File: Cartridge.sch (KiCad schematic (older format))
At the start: 1 part, among them J4 Expansion

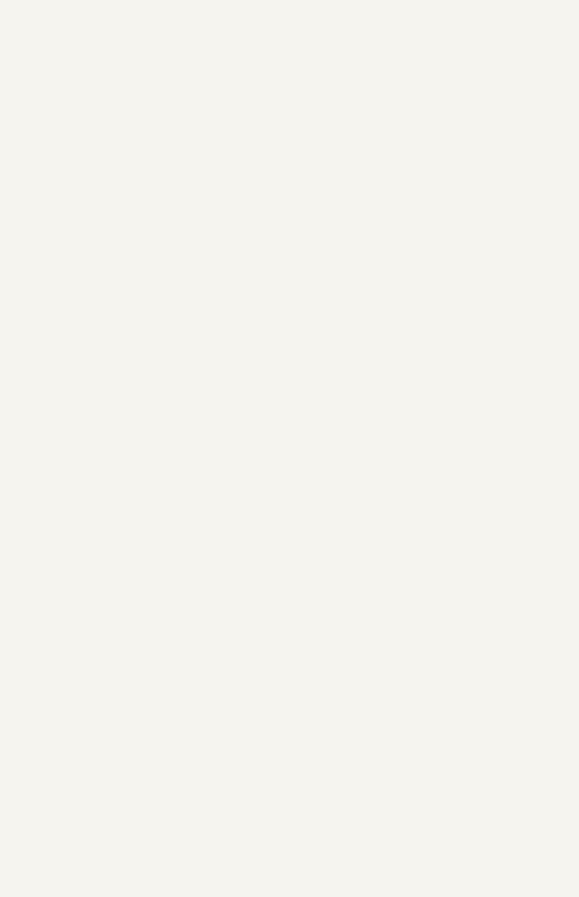
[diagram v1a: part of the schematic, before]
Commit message: MMU, Joy, Cart and Video
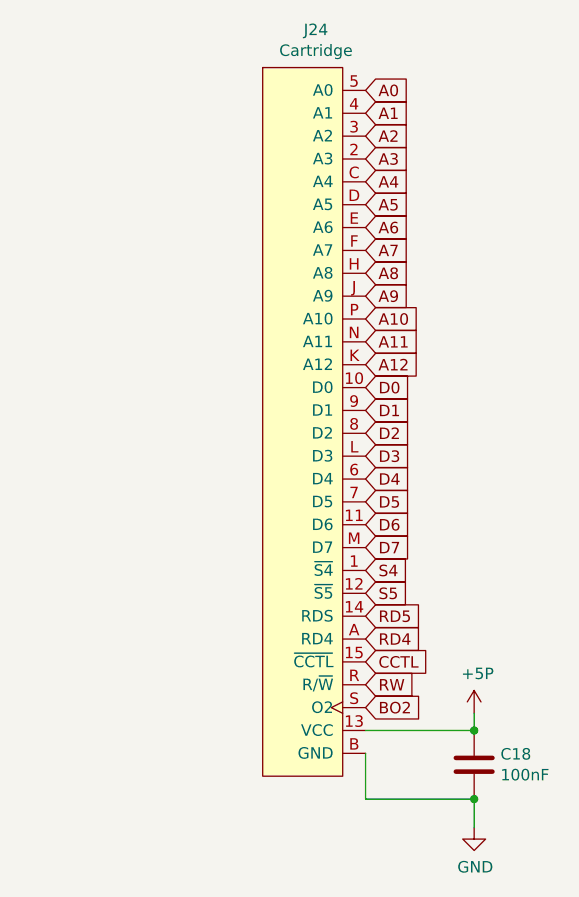
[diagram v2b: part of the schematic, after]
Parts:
- added C18: 100nF, Atari:C_Axial_L5.1mm_D2.5mm_P12.50mm_Horizontal, symbol Device:C
- added J24: Cartridge, Atari:Cartridge_Slot, symbol Atari:Cartridge
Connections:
- net GND: now also C18.2, J24.B (GND)
- new net +5P: C18.1, J24.13 (VCC)
- new net A0: J24.5 (A0)
- new net A1: J24.4 (A1)
- new net A10: J24.P (A10)
- new net A11: J24.N (A11)
- new net A12: J24.K (A12)
- new net A2: J24.3 (A2)
- new net A3: J24.2 (A3)
- new net A4: J24.C (A4)
- new net A5: J24.D (A5)
- new net A6: J24.E (A6)
- new net A7: J24.F (A7)
- new net A8: J24.H (A8)
- new net A9: J24.J (A9)
- new net BO2: J24.S (O2)
- new net CCTL: J24.15 (~CCTL)
- new net D0: J24.10 (D0)
- new net D1: J24.9 (D1)
- new net D2: J24.8 (D2)
- new net D3: J24.L (D3)
- new net D4: J24.6 (D4)
- new net D5: J24.7 (D5)
- new net D6: J24.11 (D6)
- new net D7: J24.M (D7)
- new net RD4: J24.A (RD4)
- new net RD5: J24.14 (RDS)
- new net RW: J24.R (R/~W)
- new net S4: J24.1 (~S4)
- new net S5: J24.12 (~S5)
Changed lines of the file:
@@
 $Descr A4 11693 8268
 encoding utf-8
-Sheet 7 14
+Sheet 7 15
 Title ""
 Date ""
@@
 Wire Wire Line
 	3125 3950 3125 3750
+$Comp
+L Atari:Cartridge J24
+U 1 1 602F6C5A
+P 6700 3500
+F 0 "J24" H 6783 5215 50  0000 C CNN
+F 1 "Cartridge" H 6783 5124 50  0000 C CNN
+F 2 "Atari:Cartridge_Slot" H 7100 3450 50  0001 C CNN
+F 3 "" H 7100 3450 50  0001 C CNN
+	1    6700 3500
+	1    0    0    -1
+$EndComp
+Text GLabel 7000 2050 2    50   Input ~ 0
+A0
+Text GLabel 7000 2150 2    50   Input ~ 0
+A1
+Text GLabel 7000 2250 2    50   Input ~ 0
+A2
+Text GLabel 7000 2350 2    50   Input ~ 0
+A3
+Text GLabel 7000 2450 2    50   Input ~ 0
+A4
+Text GLabel 7000 2550 2    50   Input ~ 0
+A5
+Text GLabel 7000 2650 2    50   Input ~ 0
+A6
+Text GLabel 7000 2750 2    50   Input ~ 0
+A7
+Text GLabel 7000 2850 2    50   Input ~ 0
+A8
+Text GLabel 7000 2950 2    50   Input ~ 0
+A9
+Text GLabel 7000 3050 2    50   Input ~ 0
+A10
+Text GLabel 7000 3150 2    50   Input ~ 0
+A11
+Text GLabel 7000 3250 2    50   Input ~ 0
+A12
+Text GLabel 7000 3350 2    50   Input ~ 0
+D0
+Text GLabel 7000 3450 2    50   Input ~ 0
+D1
+Text GLabel 7000 3550 2    50   Input ~ 0
+D2
+Text GLabel 7000 3650 2    50   Input ~ 0
+D3
+Text GLabel 7000 3750 2    50   Input ~ 0
+D4
+Text GLabel 7000 3850 2    50   Input ~ 0
+D5
+Text GLabel 7000 3950 2    50   Input ~ 0
+D6
+Text GLabel 7000 4050 2    50   Input ~ 0
+D7
+Text GLabel 7000 4150 2    50   Input ~ 0
+S4
+Text GLabel 7000 4250 2    50   Input ~ 0
+S5
+Text GLabel 7000 4350 2    50   Input ~ 0
+RD5
+Text GLabel 7000 4450 2    50   Input ~ 0
+RD4
+Text GLabel 7000 4550 2    50   Input ~ 0
+CCTL
+Text GLabel 7000 4650 2    50   Input ~ 0
+RW
+Text GLabel 7000 4750 2    50   Input ~ 0
+BO2
+$Comp
+L power:+5P #PWR0197
+U 1 1 602F9620
+P 7475 4775
+F 0 "#PWR0197" H 7475 4625 50  0001 C CNN
+F 1 "+5P" H 7490 4948 50  0000 C CNN
+F 2 "" H 7475 4775 50  0001 C CNN
+F 3 "" H 7475 4775 50  0001 C CNN
+	1    7475 4775
+	1    0    0    -1
+$EndComp
+$Comp
+L Device:C C18
+U 1 1 602F9DE7
+P 7475 5000
+F 0 "C18" H 7590 5046 50  0000 L CNN
+F 1 "100nF" H 7590 4955 50  0000 L CNN
+F 2 "Atari:C_Axial_L5.1mm_D2.5mm_P12.50mm_Horizontal" H 7513 4850 50  0001 C CNN
+F 3 "~" H 7475 5000 50  0001 C CNN
+	1    7475 5000
+	1    0    0    -1
+$EndComp
+Wire Wire Line
+	7000 4850 7475 4850
+Wire Wire Line
+	7475 4775 7475 4850
+Connection ~ 7475 4850
+Wire Wire Line
+	7000 4950 7000 5150
+Wire Wire Line
+	7000 5150 7475 5150
+$Comp
+L power:GND #PWR0198
+U 1 1 602FAB68
+P 7475 5275
+F 0 "#PWR0198" H 7475 5025 50  0001 C CNN
+F 1 "GND" H 7480 5102 50  0000 C CNN
+F 2 "" H 7475 5275 50  0001 C CNN
+F 3 "" H 7475 5275 50  0001 C CNN
+	1    7475 5275
+	1    0    0    -1
+$EndComp
+Wire Wire Line
+	7475 5150 7475 5275
+Connection ~ 7475 5150
 $EndSCHEMATC
